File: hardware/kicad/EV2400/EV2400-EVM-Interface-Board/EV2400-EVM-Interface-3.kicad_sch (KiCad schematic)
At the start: 36 parts, among them U10 TPS73601DBV, U11 TPS73601DBV, U12 TPS73601DBV, U13 TPS73601DBV, U14 ISL90842UIV1427Z, U15 TPS73601DBV, U18 TPS73601DBV, U9 ISL90842UIV1427Z

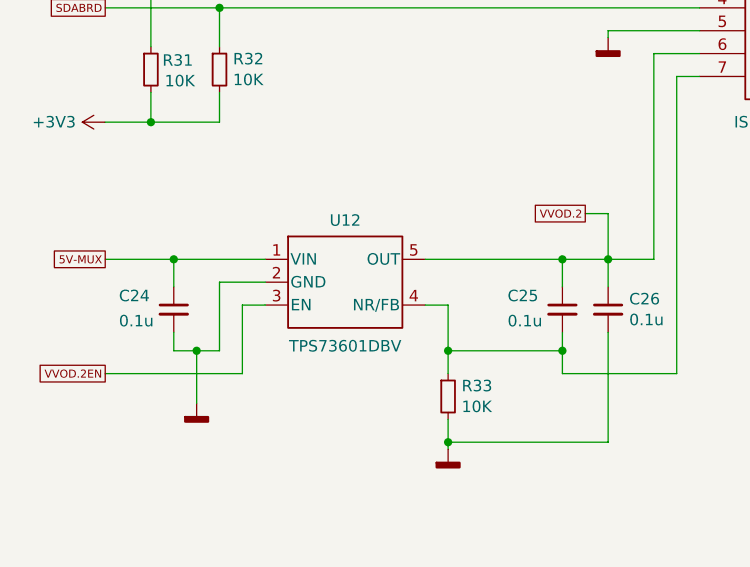
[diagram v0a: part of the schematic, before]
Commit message: Update EV2400 kicad files
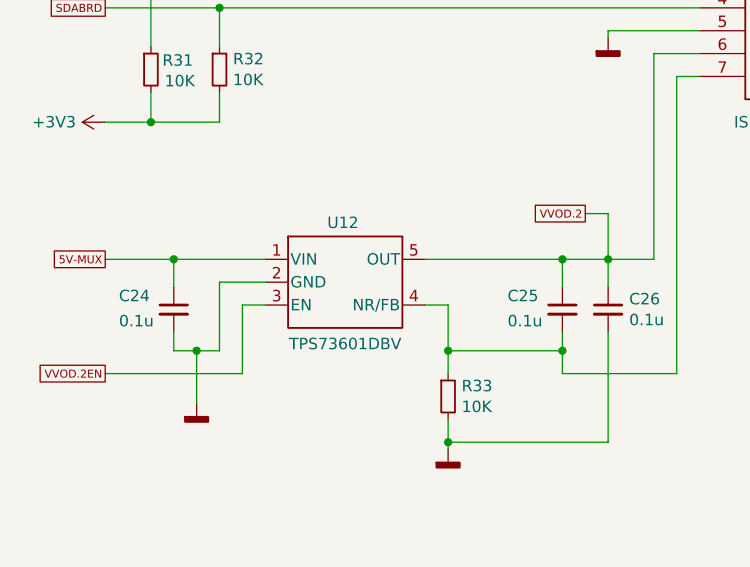
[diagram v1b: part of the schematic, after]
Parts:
- removed U12: TPS73601DBV, EV2400-Footprints:SOT95P280X145-5N, symbol EV2400-EVM-Interface-Board-rescue:TPS73601DBV-EV2400-Components
- added U12: TPS73601DBV, EV2400-Footprints:SOT95P280X145-5N, symbol EV2400-Components:TPS73601DBV
- C18, C19, C20, C21, C22, C23, C24, C25, C26, C27, C28, C29, C30, C31, C32, C33, C34, C35: symbol EV2400-EVM-Interface-Board-rescue:C_Small-EV2400-Components -> EV2400-Components:C_Small
- R29, R30, R31, R32, R33, R34, R35, R36, R37, R38: symbol EV2400-EVM-Interface-Board-rescue:R_Small-EV2400-Components -> EV2400-Components:R_Small
- U10, U11, U13, U15, U18: symbol EV2400-EVM-Interface-Board-rescue:TPS73601DBV-EV2400-Components -> EV2400-Components:TPS73601DBV; Description_1 (none) -> LDO Voltage Regulators Cap-Free NMOS 400mA
- U14, U9: symbol EV2400-EVM-Interface-Board-rescue:ISL90842-EV2400-Components -> EV2400-Components:ISL90842; Description_1 (none) -> Digital Potentiometer ICs ISL90842UIV1427Z LW NOISE LW PWR 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
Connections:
- net 5V-MUX: now also U12.1 (VIN)
- net GND: now also U12.2 (GND)
- net VVOD.2: now also U12.5 (OUT)
- net VVOD.2EN: now also U12.3 (EN)
- net at C25.2, R33.1, U9.7 (RH2): now also U12.4 (NR/FB)
